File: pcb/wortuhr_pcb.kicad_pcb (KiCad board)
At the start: 2 copper layers, 73.4 x 42.6 mm, 36 parts, among them J1 Conn_01x05_Male, J2 Conn_01x03_Male, SW1 SW_Push, SW2 SW_Push, SW3 SW_Push, U1 LM1117-3.3, U2 ESP-12F, X1 250-x02

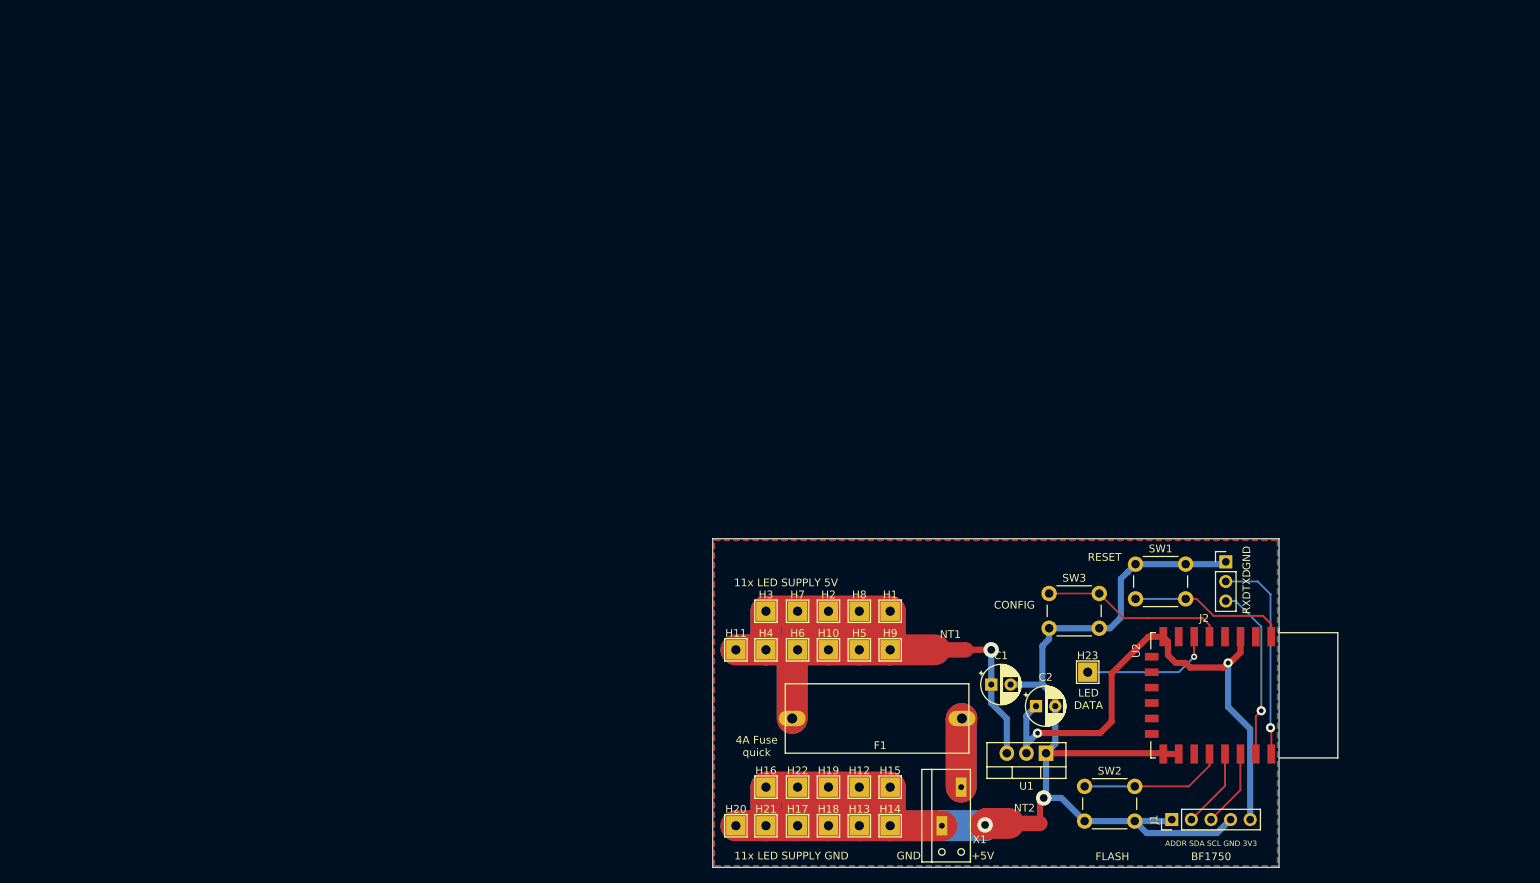
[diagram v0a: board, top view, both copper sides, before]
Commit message: New PCB V2
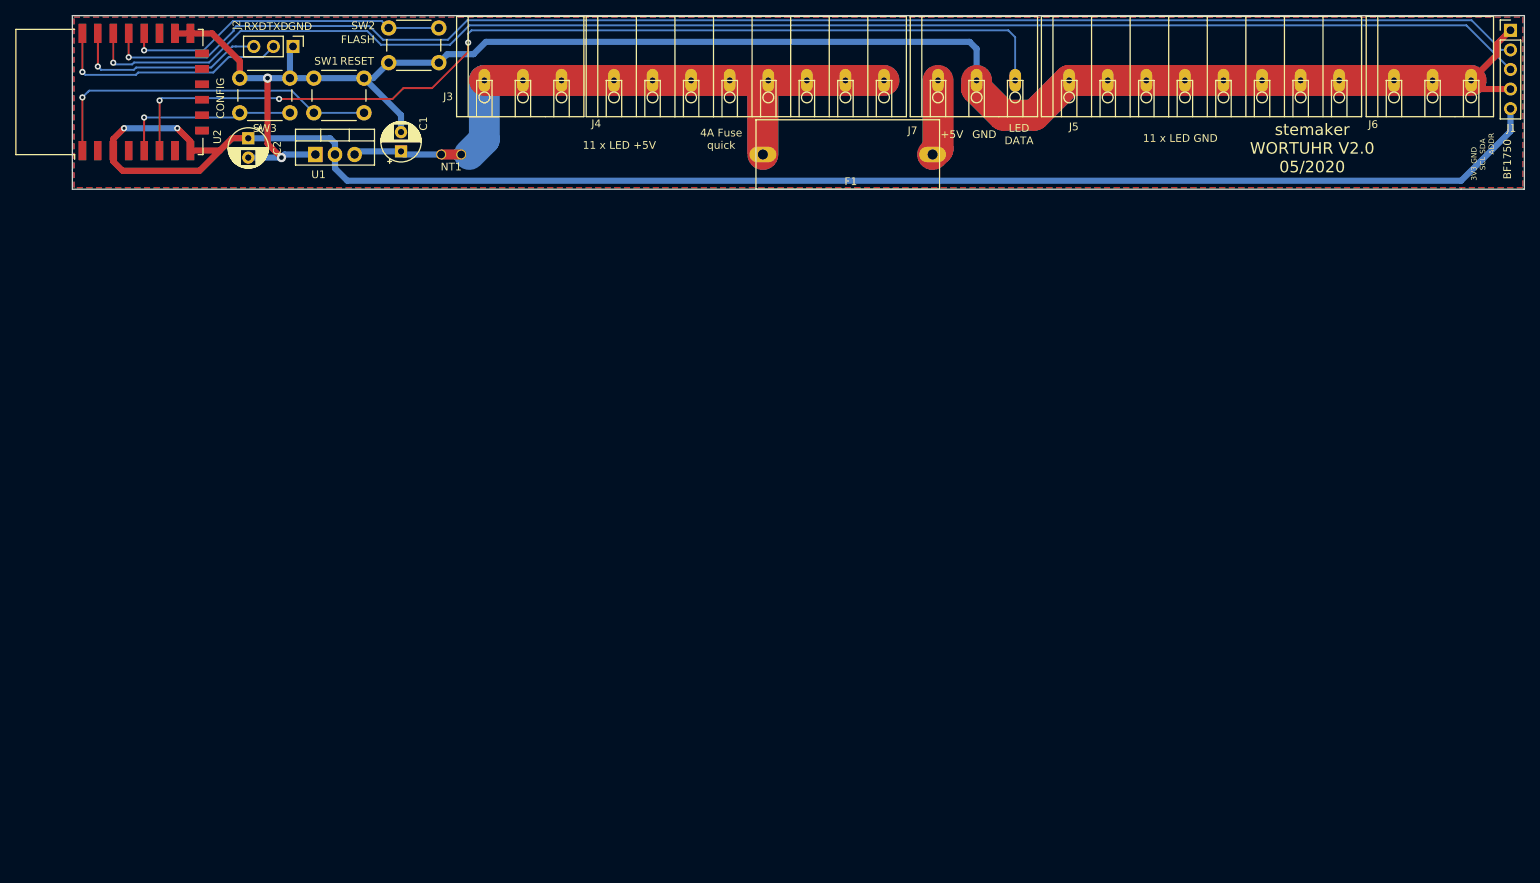
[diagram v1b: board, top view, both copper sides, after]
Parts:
- removed H1, H10, H11, H12, H13, H14, H15, H16, H17, H18, H19, H2, H20, H21, H22, H23, H3, H4, H5, H6, H7, H8, H9: MountingHole_Pad, TestPoint:TestPoint_THTPad_2.5x2.5mm_Drill1.2mm
- removed NT2: Net-Tie_2, NetTie:NetTie-2_SMD_Pad2.0mm
- removed X1: 250-x02, stemaker_connectoren:WAGO_250-402
- added J3: Conn_01x03_Male, stemaker_connectoren:WAGO_250-503, F.Cu at (79.8, 43.1)
- added J4: Conn_01x08_Male, stemaker_connectoren:WAGO_250-508, F.Cu at (96.6, 43.1)
- added J5: Conn_01x08_Male, stemaker_connectoren:WAGO_250-508, F.Cu at (155.6, 43.1)
- added J6: Conn_01x03_Male, stemaker_connectoren:WAGO_250-503, F.Cu at (197.7, 43.1)
- added J7: Conn_01x03_Male, stemaker_connectoren:WAGO_250-503, F.Cu at (138.6, 43.1)
- NT1: footprint NetTie:NetTie-2_SMD_Pad2.0mm -> NetTie:NetTie-2_THT_Pad1.0mm
- moved U2 166.6 mm to (34.8, 39.9), turned to 90 degrees
- moved J2 138.1 mm to (58.6, 34.0), turned to 270 degrees
- moved SW2 133.4 mm to (71.0, 31.6)
- moved C2 125.9 mm to (52.8, 45.9), turned to 270 degrees
- moved SW1 123.7 mm to (61.3, 38.1)
- moved U1 122.4 mm to (61.5, 48.0), turned to 0 degrees
- moved SW3 116.5 mm to (58.2, 42.6), turned to 180 degrees
- moved J1 111.3 mm to (216.4, 31.9), turned to 0 degrees
- moved C1 103.1 mm to (72.6, 47.6), turned to 90 degrees
- moved NT1 90.2 mm to (80.4, 48.0), turned to 180 degrees
- moved F1 73.2 mm to (119.5, 48.0)
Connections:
- net Net-(J2-Pad2) renamed /TXD
- net Net-(J2-Pad3) renamed /RXD
- net Net-(SW1-Pad2) renamed /RESET
- net Net-(SW2-Pad1) renamed /FLASH
- net Net-(SW3-Pad1) renamed /CFG
- U2 pad 6: Net-(H23-Pad1) -> /LED_DATA
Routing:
- net GND: track 109.7 -> 298.8 mm, vias 1 -> 2
- net /SCL: track 10.1 -> 190.9 mm, vias 0 -> 1
- net /SDA: track 10.3 -> 187.7 mm, vias 0 -> 1
- net /LED_GND: track 144.4 -> 0.00 mm, vias 1 -> 0
- net +3V3: track 71.7 -> 212.3 mm
- net /LED_DATA: track 0.00 -> 128.6 mm, vias 0 -> 3
- net /RESET: track 20.6 -> 45.0 mm, vias 0 -> 1
- net /FLASH: track 18.8 -> 42.3 mm, vias 0 -> 1
- net Net-(H23-Pad1): track 17.2 -> 0.00 mm, vias 1 -> 0
- net /LED_5V: track 146.4 -> 133.8 mm
- net +5V: track 17.5 -> 11.6 mm, vias 1 -> 0
- net /TXD: track 27.2 -> 31.4 mm
- net /RXD: track 22.8 -> 25.9 mm
- net /MAIN_SUPPLY: track 17.9 -> 19.8 mm
- net /CFG: track 24.3 -> 23.4 mm, vias 0 -> 1
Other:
- board size 73.4 x 42.6 mm -> 188.2 x 22.5 mm
- board text added: "11 x LED +5V"
- board text added: "11 x LED GND"
- board text added: "3V3 GND SCL SDA ADDR"
- board text added: "stemaker WORTUHR V2.0 05/2020"
- board text removed: "11x LED SUPPLY 5V"
- board text removed: "11x LED SUPPLY GND"
- board text removed: "ADDR SDA SCL GND 3V3"
